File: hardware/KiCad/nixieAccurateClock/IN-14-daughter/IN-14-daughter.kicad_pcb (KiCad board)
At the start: 4 copper layers, 19 x 32 mm, 12 parts, among them J1 Conn_02x05_Odd_Even, U1 HV509K6-G

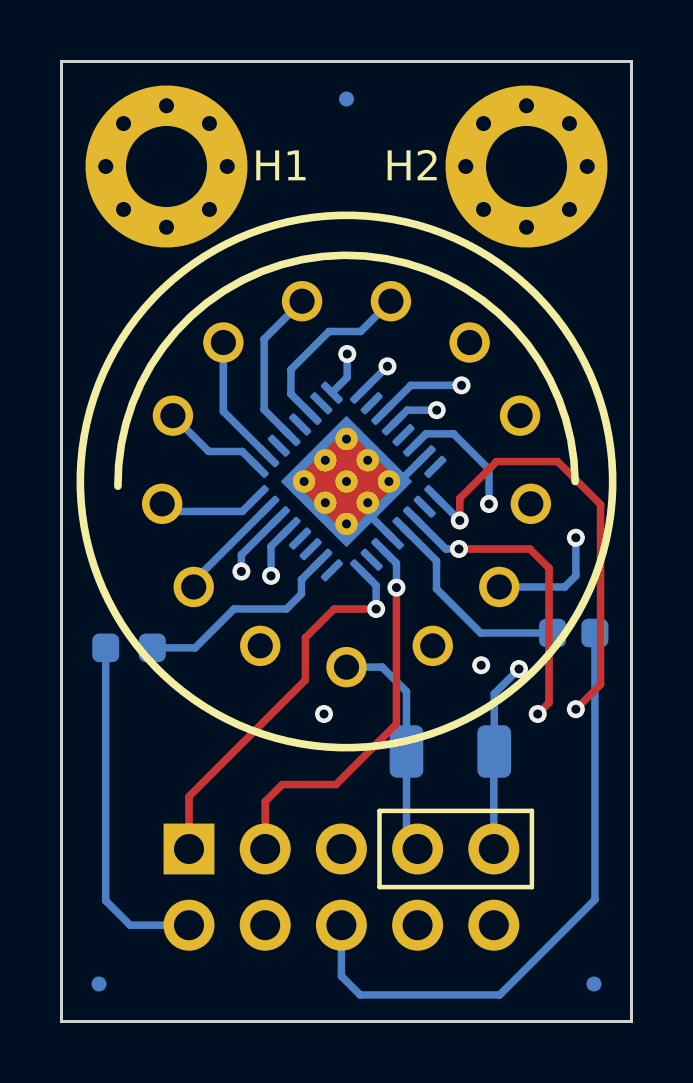
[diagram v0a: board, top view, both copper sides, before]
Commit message: add thermal reliefs
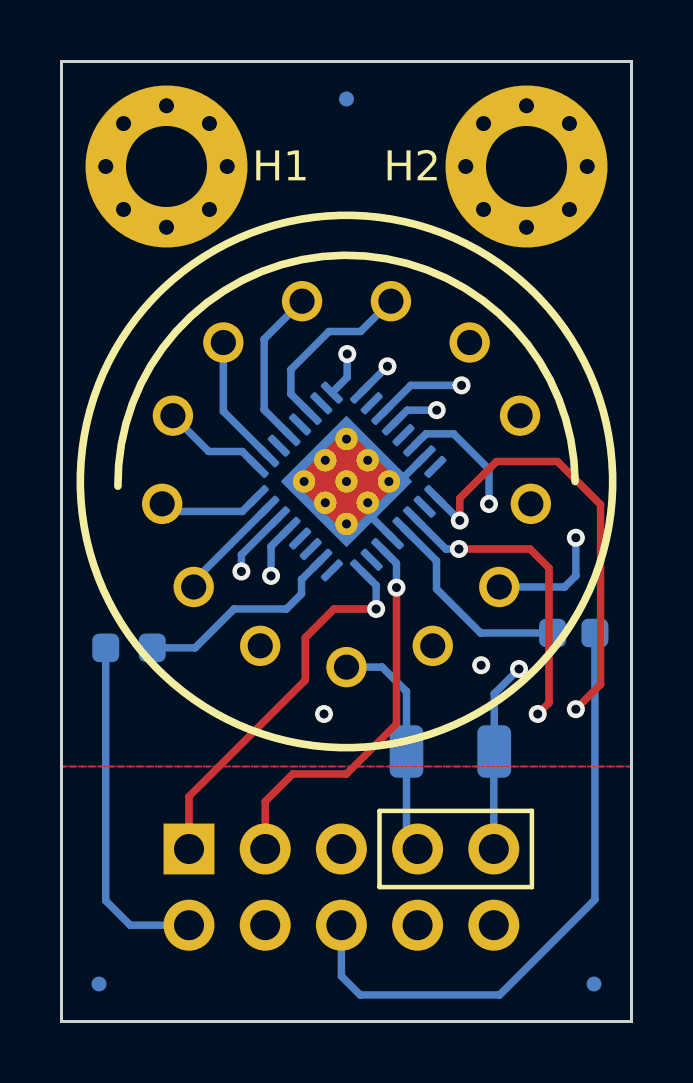
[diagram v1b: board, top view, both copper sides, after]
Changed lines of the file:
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@@
   (segment (start 43.503903 31.068243) (end 44.56066 32.125) (width 0.25) (layer "B.Cu") (net 33))
   (segment (start 45 32.125) (end 44.56066 32.125) (width 0.25) (layer "B.Cu") (net 33))
-  (segment (start 40.896446 39.978554) (end 42.915725 37.959275) (width 0.25) (layer "F.Cu") (net 34))
-  (segment (start 39.103553 39.978554) (end 38.54 40.542107) (width 0.25) (layer "F.Cu") (net 34))
+  (segment (start 39.457107 39.625) (end 38.54 40.542107) (width 0.25) (layer "F.Cu") (net 34))
+  (segment (start 42.915725 33.411533) (end 42.915725 37.959275) (width 0.25) (layer "F.Cu") (net 34))
+  (segment (start 42.915725 37.959275) (end 41.25 39.625) (width 0.25) (layer "F.Cu") (net 34))
+  (segment (start 41.25 39.625) (end 39.457107 39.625) (width 0.25) (layer "F.Cu") (net 34))
   (segment (start 38.54 40.542107) (end 38.54 42.125) (width 0.25) (layer "F.Cu") (net 34))
-  (segment (start 40.896446 39.978554) (end 39.103553 39.978554) (width 0.25) (layer "F.Cu") (net 34))
-  (segment (start 42.915725 33.411533) (end 42.915725 37.959275) (width 0.25) (layer "F.Cu") (net 34))
   (via (at 42.915725 33.411533) (size 0.6) (drill 0.3) (layers "F.Cu" "B.Cu") (net 34))
   (segment (start 42.769278 32.454938) (end 42.443243 32.128903) (width 0.25) (layer "B.Cu") (net 34))
   (segment (start 42.915725 33.411533) (end 42.915725 32.601385) (width 0.25) (layer "B.Cu") (net 34))
   (segment (start 42.915725 32.601385) (end 42.769278 32.454938) (width 0.25) (layer "B.Cu") (net 34))
+  (zone (net 3) (net_name "GND") (layers "F.Cu" "In1.Cu" "In2.Cu" "B.Cu") (hatch edge 0.5)
+    (priority 1)
+    (connect_pads (clearance 0.5))
+    (min_thickness 0.25) (filled_areas_thickness no)
+    (fill (thermal_gap 0.5) (thermal_bridge_width 0.5))
+    (polygon
+      (pts
+        (xy 31.75 47.875)
+        (xy 31.75 39.375)
+        (xy 50.75 39.375)
+        (xy 50.75 47.875)
+      )
+    )
+  )
   (zone (net 3) (net_name "GND") (layers "F.Cu" "In1.Cu" "In2.Cu" "B.Cu") (hatch edge 0.5)
     (connect_pads yes (clearance 0.5))
@@
         (xy 31.75 15.875)
         (xy 50.75 15.875)
-        (xy 50.75 47.875)
-        (xy 31.75 47.875)
+        (xy 50.75 39.375)
+        (xy 31.75 39.375)
       )
     )
